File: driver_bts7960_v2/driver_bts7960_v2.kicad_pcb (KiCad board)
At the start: 2 copper layers, 56.4 x 42.1 mm, 31 parts, among them J1 Motor_1, J2 Alimentacion, J6 Motor_2, J7 Conn_02x04_Odd_Even, U1 BTS7960B, U2 BTS7960B, U3 BTS7960B, U4 BTS7960B

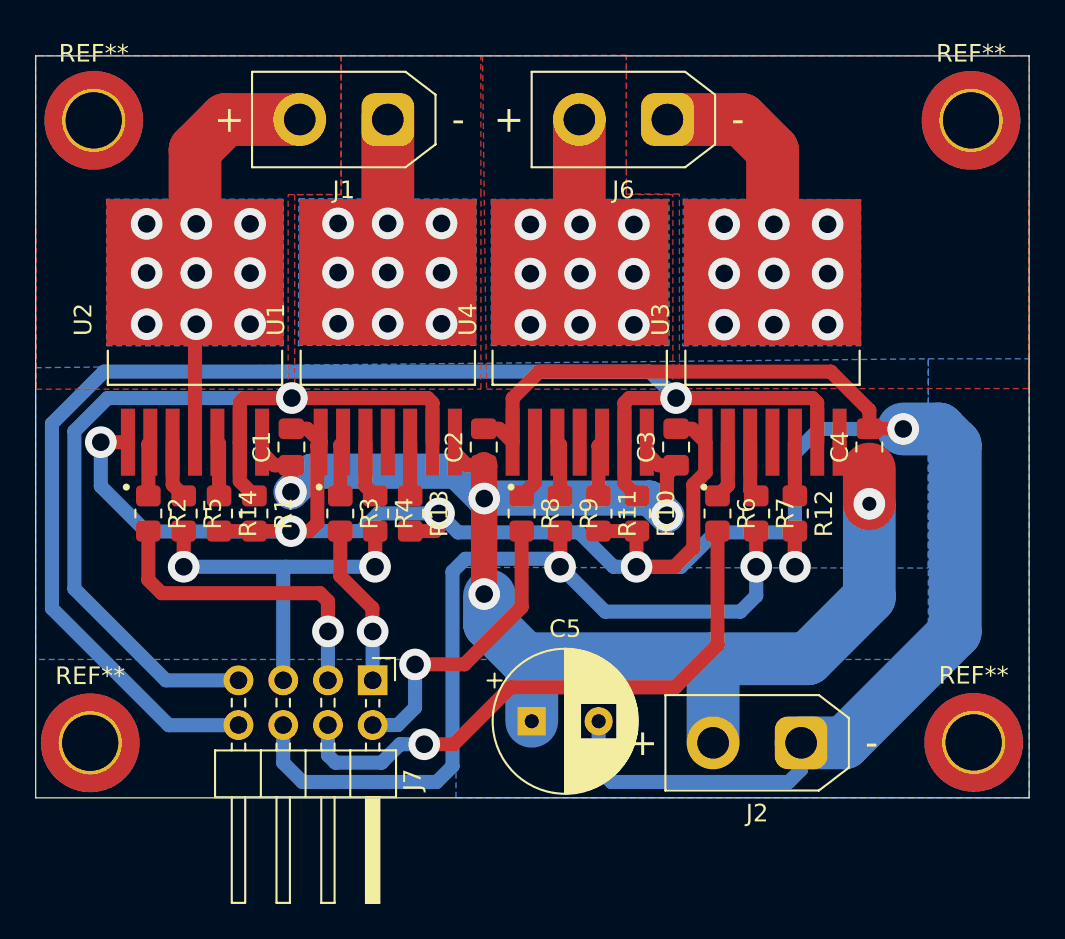
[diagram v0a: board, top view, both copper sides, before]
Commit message: .
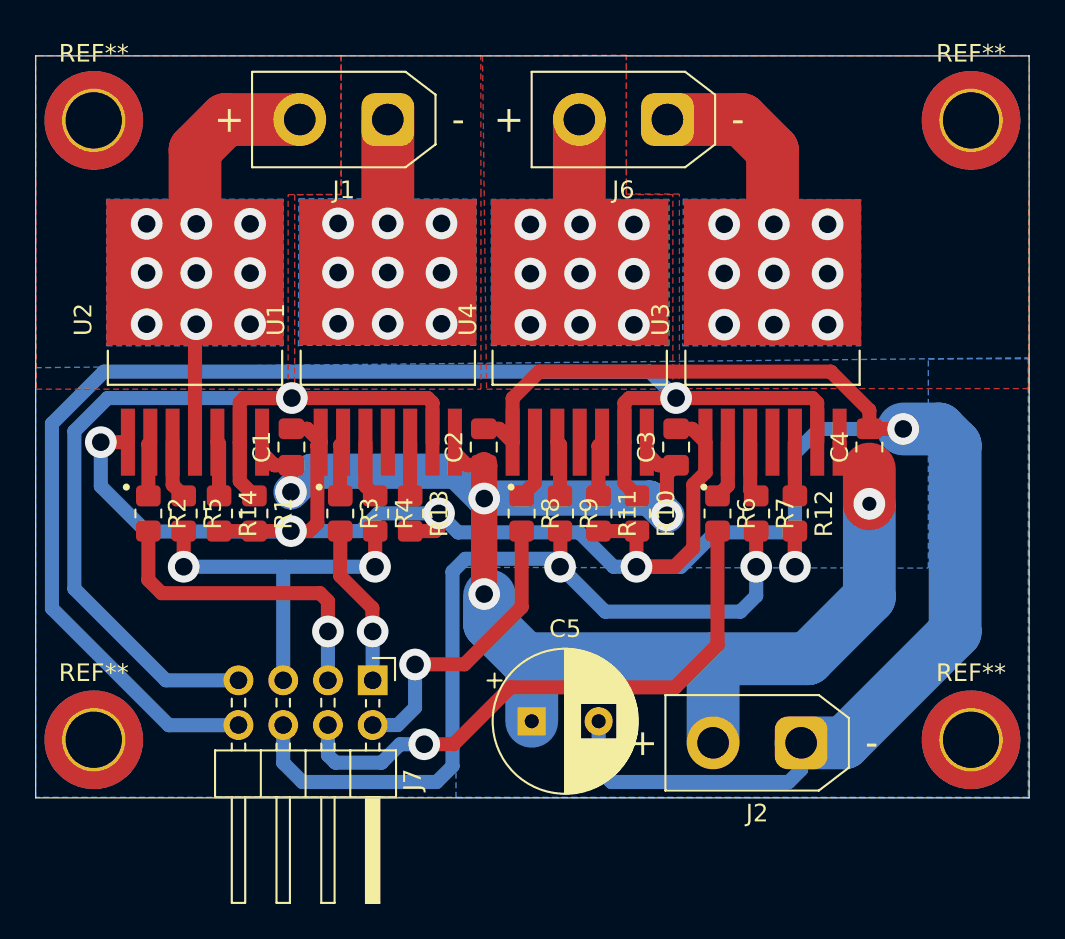
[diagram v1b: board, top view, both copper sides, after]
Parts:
- moved REF** 0.27 mm to (111.9, 73.6)
- moved REF** 0.21 mm to (161.7, 73.6)
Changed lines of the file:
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@@
 	(footprint "MountingHole:MountingHole_3.2mm_M3_DIN965_Pad_TopBottom"
 		(layer "F.Cu")
-		(at 111.7 73.775)
+		(at 111.9 73.6)
 		(descr "Mounting Hole 3.2mm, M3, DIN965")
 		(tags "mounting hole 3.2mm m3 din965")
@@
 	(footprint "MountingHole:MountingHole_3.2mm_M3_DIN965_Pad_TopBottom"
 		(layer "F.Cu")
-		(at 161.875 73.75)
+		(at 161.725 73.6)
 		(descr "Mounting Hole 3.2mm, M3, DIN965")
 		(tags "mounting hole 3.2mm m3 din965")
@@
 		(polygon
 			(pts
-				(xy 108.6 52.4695) (xy 159.3 51.963674) (xy 159.3 69.04) (xy 108.6 69.04)
+				(xy 108.6 52.4695) (xy 164.975 51.907056) (xy 164.975 76.87) (xy 108.6 76.87)
 			)
 		)
